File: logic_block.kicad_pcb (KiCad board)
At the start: 2 copper layers, 40 x 40 mm, 33 parts, among them J301 PogoPin, J302 PogoPin, J303 PogoPin, J304 PogoPin, J305 PogoPin, J306 PogoPin, J307 WritePad, Q301 NMOS, Q302 NMOS, Q303 NMOS, Q304 NMOS, U301 ATtiny404-SS

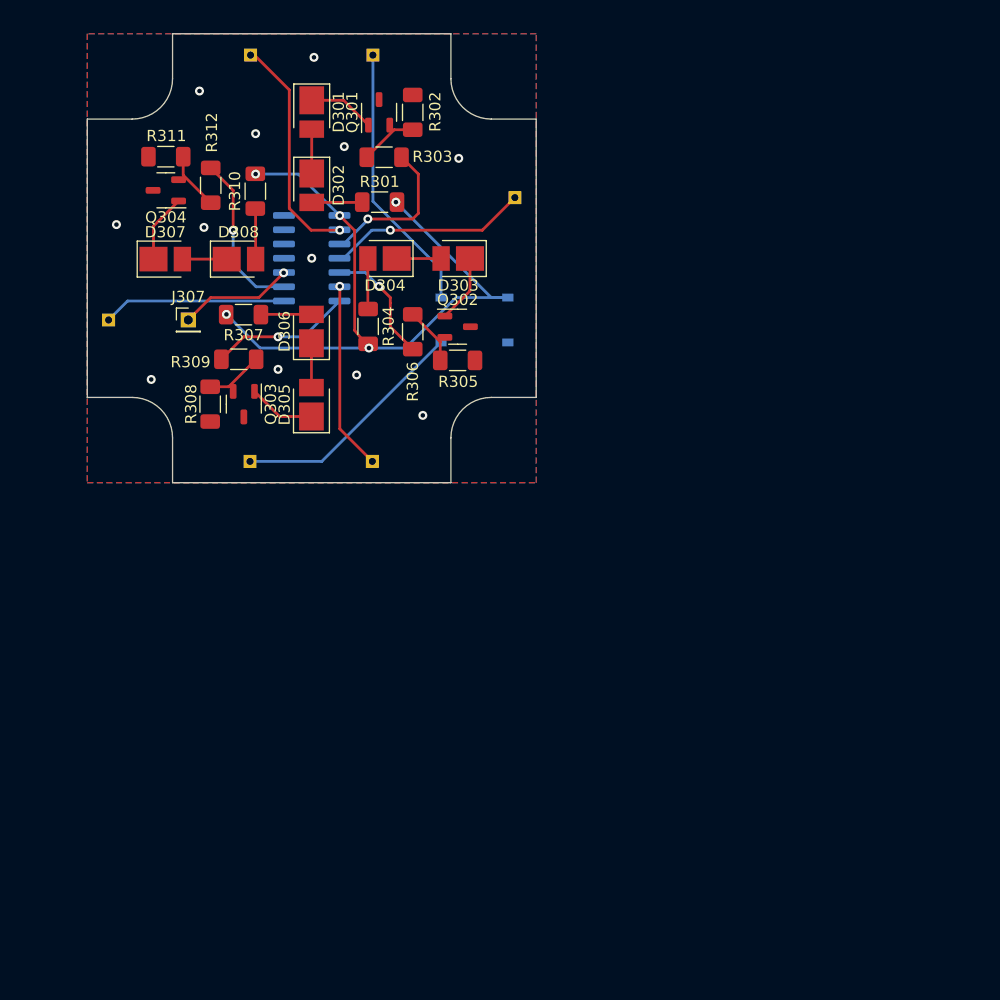
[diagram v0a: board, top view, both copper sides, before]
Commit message: gerber
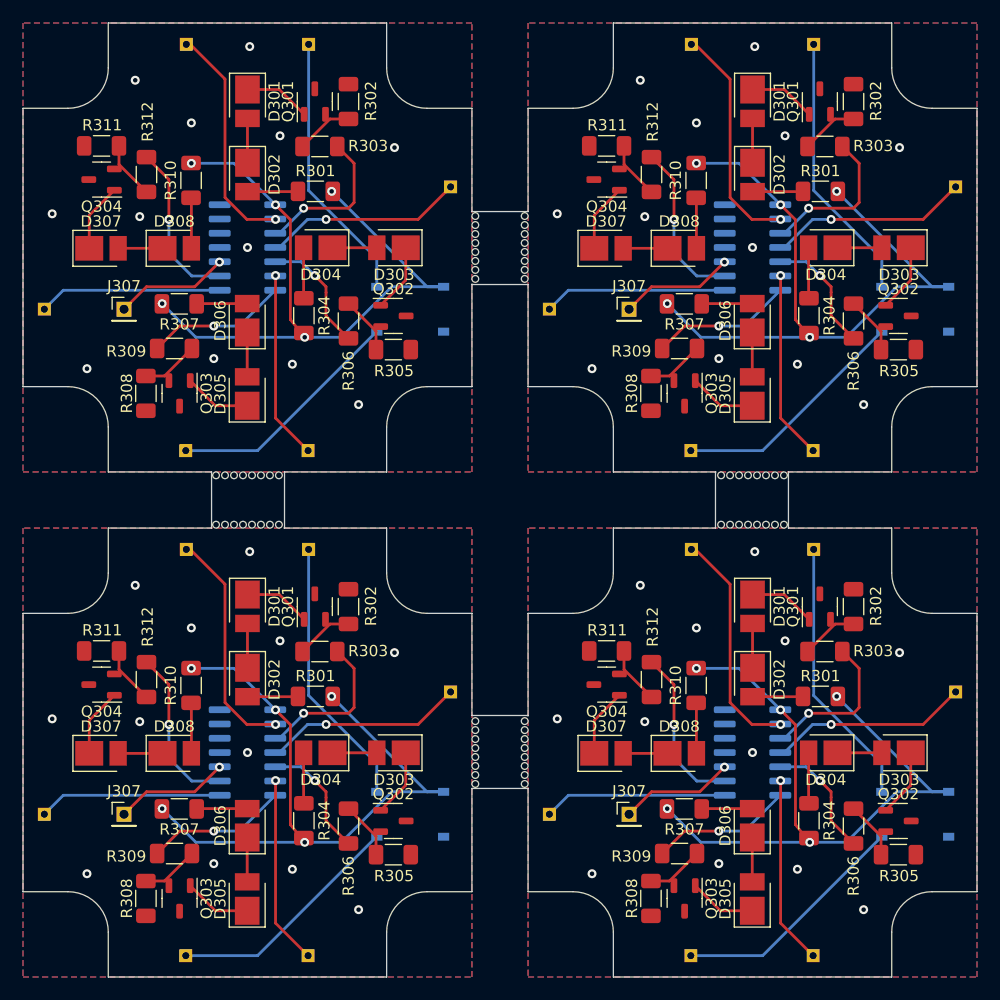
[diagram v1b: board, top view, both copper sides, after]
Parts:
- removed the D301 at (120.0, 57.0)
- removed the D302 at (120.0, 63.5)
- removed the D303 at (133.1, 70.0)
- removed the D304 at (126.5, 70.0)
- removed the D305 at (120.0, 83.0)
- removed the D306 at (120.0, 76.5)
- removed the D307 at (107.0, 70.1)
- removed the D308 at (113.5, 70.1)
- removed the D309 at (134.5, 75.5)
- removed the J301 at (114.5, 51.9)
- removed the J302 at (138.1, 64.6)
- removed the J303 at (125.4, 88.1)
- removed the J304 at (101.9, 75.5)
- removed the J305 at (125.5, 51.9)
- removed the J306 at (114.5, 88.1)
- removed the J307 at (109.0, 75.5)
- removed the Q301 at (126.0, 57.0)
- removed the Q302 at (133.0, 76.1)
- removed the Q303 at (114.0, 83.0)
- removed the Q304 at (107.0, 64.0)
- removed the R301 at (126.0, 65.0)
- removed the R302 at (129.0, 57.0)
- removed the R303 at (126.5, 61.0)
- removed the R304 at (125.0, 76.1)
- removed the R305 at (133.0, 79.1)
- removed the R306 at (129.0, 76.5)
- removed the R307 at (113.9, 75.0)
- removed the R308 at (111.0, 83.0)
- removed the R309 at (113.5, 79.0)
- removed the R310 at (115.0, 64.0)
- removed the R311 at (107.0, 61.0)
- removed the R312 at (111.0, 63.5)
- removed the U301 at (120.0, 70.0)
- added D301: LED, LED_SMD:LED_PLCC_2835_Handsoldering, F.Cu at (114.3, 56.0)
- added D301: LED, LED_SMD:LED_PLCC_2835_Handsoldering, F.Cu at (114.3, 101.0)
- added D301: LED, LED_SMD:LED_PLCC_2835_Handsoldering, F.Cu at (159.3, 56.0)
- added D301: LED, LED_SMD:LED_PLCC_2835_Handsoldering, F.Cu at (159.3, 101.0)
- added D302: LED, LED_SMD:LED_PLCC_2835_Handsoldering, F.Cu at (159.3, 62.5)
- added D302: LED, LED_SMD:LED_PLCC_2835_Handsoldering, F.Cu at (114.3, 107.5)
- added D302: LED, LED_SMD:LED_PLCC_2835_Handsoldering, F.Cu at (114.3, 62.5)
- added D302: LED, LED_SMD:LED_PLCC_2835_Handsoldering, F.Cu at (159.3, 107.5)
- added D303: LED, LED_SMD:LED_PLCC_2835_Handsoldering, F.Cu at (172.3, 69.1)
- added D303: LED, LED_SMD:LED_PLCC_2835_Handsoldering, F.Cu at (127.3, 69.1)
- added D303: LED, LED_SMD:LED_PLCC_2835_Handsoldering, F.Cu at (127.3, 114.1)
- added D303: LED, LED_SMD:LED_PLCC_2835_Handsoldering, F.Cu at (172.3, 114.1)
- added D304: LED, LED_SMD:LED_PLCC_2835_Handsoldering, F.Cu at (165.8, 114.1)
- added D304: LED, LED_SMD:LED_PLCC_2835_Handsoldering, F.Cu at (120.8, 114.1)
- added D304: LED, LED_SMD:LED_PLCC_2835_Handsoldering, F.Cu at (165.8, 69.1)
- added D304: LED, LED_SMD:LED_PLCC_2835_Handsoldering, F.Cu at (120.8, 69.1)
- added D305: LED, LED_SMD:LED_PLCC_2835_Handsoldering, F.Cu at (159.2, 82.1)
- added D305: LED, LED_SMD:LED_PLCC_2835_Handsoldering, F.Cu at (159.2, 127.1)
- added D305: LED, LED_SMD:LED_PLCC_2835_Handsoldering, F.Cu at (114.2, 82.1)
- added D305: LED, LED_SMD:LED_PLCC_2835_Handsoldering, F.Cu at (114.2, 127.1)
- added D306: LED, LED_SMD:LED_PLCC_2835_Handsoldering, F.Cu at (159.2, 120.6)
- added D306: LED, LED_SMD:LED_PLCC_2835_Handsoldering, F.Cu at (159.2, 75.6)
- added D306: LED, LED_SMD:LED_PLCC_2835_Handsoldering, F.Cu at (114.2, 75.6)
- added D306: LED, LED_SMD:LED_PLCC_2835_Handsoldering, F.Cu at (114.2, 120.6)
- added D307: LED, LED_SMD:LED_PLCC_2835_Handsoldering, F.Cu at (101.2, 69.1)
- added D307: LED, LED_SMD:LED_PLCC_2835_Handsoldering, F.Cu at (146.2, 69.1)
- added D307: LED, LED_SMD:LED_PLCC_2835_Handsoldering, F.Cu at (101.2, 114.1)
- added D307: LED, LED_SMD:LED_PLCC_2835_Handsoldering, F.Cu at (146.2, 114.1)
- added D308: LED, LED_SMD:LED_PLCC_2835_Handsoldering, F.Cu at (107.8, 114.1)
- added D308: LED, LED_SMD:LED_PLCC_2835_Handsoldering, F.Cu at (152.8, 114.1)
- added D308: LED, LED_SMD:LED_PLCC_2835_Handsoldering, F.Cu at (107.8, 69.1)
- added D308: LED, LED_SMD:LED_PLCC_2835_Handsoldering, F.Cu at (152.8, 69.1)
- added D309: ABS2, Diode_SMD:Diode_Bridge_Diotec_ABS, B.Cu at (173.8, 74.5)
- added D309: ABS2, Diode_SMD:Diode_Bridge_Diotec_ABS, B.Cu at (128.8, 74.5)
- added D309: ABS2, Diode_SMD:Diode_Bridge_Diotec_ABS, B.Cu at (173.8, 119.5)
- added D309: ABS2, Diode_SMD:Diode_Bridge_Diotec_ABS, B.Cu at (128.8, 119.5)
- added J301: PogoPin, LIB:0906015207614110, B.Cu at (108.8, 50.9)
- added J301: PogoPin, LIB:0906015207614110, B.Cu at (108.8, 95.9)
- added J301: PogoPin, LIB:0906015207614110, B.Cu at (153.8, 50.9)
- added J301: PogoPin, LIB:0906015207614110, B.Cu at (153.8, 95.9)
- added J302: PogoPin, LIB:0906015207614110, B.Cu at (177.4, 108.6)
- added J302: PogoPin, LIB:0906015207614110, B.Cu at (132.4, 63.6)
- added J302: PogoPin, LIB:0906015207614110, B.Cu at (177.4, 63.6)
- added J302: PogoPin, LIB:0906015207614110, B.Cu at (132.4, 108.6)
- added J303: PogoPin, LIB:0906015207614110, B.Cu at (119.7, 132.1)
- added J303: PogoPin, LIB:0906015207614110, B.Cu at (164.7, 132.1)
- added J303: PogoPin, LIB:0906015207614110, B.Cu at (164.7, 87.1)
- added J303: PogoPin, LIB:0906015207614110, B.Cu at (119.7, 87.1)
- added J304: PogoPin, LIB:0906015207614110, B.Cu at (96.2, 119.5)
- added J304: PogoPin, LIB:0906015207614110, B.Cu at (96.2, 74.5)
- added J304: PogoPin, LIB:0906015207614110, B.Cu at (141.2, 74.5)
- added J304: PogoPin, LIB:0906015207614110, B.Cu at (141.2, 119.5)
- added J305: PogoPin, LIB:0906015207614110, B.Cu at (164.7, 50.9)
- added J305: PogoPin, LIB:0906015207614110, B.Cu at (119.7, 50.9)
- added J305: PogoPin, LIB:0906015207614110, B.Cu at (164.7, 95.9)
- added J305: PogoPin, LIB:0906015207614110, B.Cu at (119.7, 95.9)
- added J306: PogoPin, LIB:0906015207614110, B.Cu at (153.8, 132.1)
- added J306: PogoPin, LIB:0906015207614110, B.Cu at (153.8, 87.1)
- added J306: PogoPin, LIB:0906015207614110, B.Cu at (108.8, 87.1)
- added J306: PogoPin, LIB:0906015207614110, B.Cu at (108.8, 132.1)
- added J307: WritePad, Connector_PinHeader_2.00mm:PinHeader_1x01_P2.00mm_Vertical, F.Cu at (103.3, 74.5)
- added J307: WritePad, Connector_PinHeader_2.00mm:PinHeader_1x01_P2.00mm_Vertical, F.Cu at (148.3, 119.5)
- added J307: WritePad, Connector_PinHeader_2.00mm:PinHeader_1x01_P2.00mm_Vertical, F.Cu at (148.3, 74.5)
- added J307: WritePad, Connector_PinHeader_2.00mm:PinHeader_1x01_P2.00mm_Vertical, F.Cu at (103.3, 119.5)
- added Q301: NMOS, Package_TO_SOT_SMD:SOT-23-3, F.Cu at (120.3, 101.0)
- added Q301: NMOS, Package_TO_SOT_SMD:SOT-23-3, F.Cu at (165.3, 56.0)
- added Q301: NMOS, Package_TO_SOT_SMD:SOT-23-3, F.Cu at (165.3, 101.0)
- added Q301: NMOS, Package_TO_SOT_SMD:SOT-23-3, F.Cu at (120.3, 56.0)
- added Q302: NMOS, Package_TO_SOT_SMD:SOT-23-3, F.Cu at (127.3, 120.1)
- added Q302: NMOS, Package_TO_SOT_SMD:SOT-23-3, F.Cu at (172.3, 75.1)
- added Q302: NMOS, Package_TO_SOT_SMD:SOT-23-3, F.Cu at (127.3, 75.1)
- added Q302: NMOS, Package_TO_SOT_SMD:SOT-23-3, F.Cu at (172.3, 120.1)
- added Q303: NMOS, Package_TO_SOT_SMD:SOT-23-3, F.Cu at (108.2, 82.0)
- added Q303: NMOS, Package_TO_SOT_SMD:SOT-23-3, F.Cu at (153.2, 82.0)
- added Q303: NMOS, Package_TO_SOT_SMD:SOT-23-3, F.Cu at (153.2, 127.0)
- added Q303: NMOS, Package_TO_SOT_SMD:SOT-23-3, F.Cu at (108.2, 127.0)
- added Q304: NMOS, Package_TO_SOT_SMD:SOT-23-3, F.Cu at (101.3, 108.0)
- added Q304: NMOS, Package_TO_SOT_SMD:SOT-23-3, F.Cu at (101.3, 63.0)
- added Q304: NMOS, Package_TO_SOT_SMD:SOT-23-3, F.Cu at (146.3, 63.0)
- added Q304: NMOS, Package_TO_SOT_SMD:SOT-23-3, F.Cu at (146.3, 108.0)
- added R301: 47Ω, Resistor_SMD:R_1206_3216Metric_Pad1.30x1.75mm_HandSolder, F.Cu at (165.3, 64.0)
- added R301: 47Ω, Resistor_SMD:R_1206_3216Metric_Pad1.30x1.75mm_HandSolder, F.Cu at (165.3, 109.0)
- added R301: 47Ω, Resistor_SMD:R_1206_3216Metric_Pad1.30x1.75mm_HandSolder, F.Cu at (120.3, 64.0)
- added R301: 47Ω, Resistor_SMD:R_1206_3216Metric_Pad1.30x1.75mm_HandSolder, F.Cu at (120.3, 109.0)
- added R302: 10kΩ, Resistor_SMD:R_1206_3216Metric_Pad1.30x1.75mm_HandSolder, F.Cu at (168.3, 101.0)
- added R302: 10kΩ, Resistor_SMD:R_1206_3216Metric_Pad1.30x1.75mm_HandSolder, F.Cu at (123.3, 56.0)
- added R302: 10kΩ, Resistor_SMD:R_1206_3216Metric_Pad1.30x1.75mm_HandSolder, F.Cu at (123.3, 101.0)
- added R302: 10kΩ, Resistor_SMD:R_1206_3216Metric_Pad1.30x1.75mm_HandSolder, F.Cu at (168.3, 56.0)
- added R303: 100Ω, Resistor_SMD:R_1206_3216Metric_Pad1.30x1.75mm_HandSolder, F.Cu at (165.7, 105.0)
- added R303: 100Ω, Resistor_SMD:R_1206_3216Metric_Pad1.30x1.75mm_HandSolder, F.Cu at (120.7, 105.0)
- added R303: 100Ω, Resistor_SMD:R_1206_3216Metric_Pad1.30x1.75mm_HandSolder, F.Cu at (120.7, 60.0)
- added R303: 100Ω, Resistor_SMD:R_1206_3216Metric_Pad1.30x1.75mm_HandSolder, F.Cu at (165.7, 60.0)
- added R304: 47Ω, Resistor_SMD:R_1206_3216Metric_Pad1.30x1.75mm_HandSolder, F.Cu at (119.3, 75.1)
- added R304: 47Ω, Resistor_SMD:R_1206_3216Metric_Pad1.30x1.75mm_HandSolder, F.Cu at (164.3, 75.1)
- added R304: 47Ω, Resistor_SMD:R_1206_3216Metric_Pad1.30x1.75mm_HandSolder, F.Cu at (164.3, 120.1)
- added R304: 47Ω, Resistor_SMD:R_1206_3216Metric_Pad1.30x1.75mm_HandSolder, F.Cu at (119.3, 120.1)
- added R305: 10kΩ, Resistor_SMD:R_1206_3216Metric_Pad1.30x1.75mm_HandSolder, F.Cu at (127.3, 78.1)
- added R305: 10kΩ, Resistor_SMD:R_1206_3216Metric_Pad1.30x1.75mm_HandSolder, F.Cu at (172.3, 78.1)
- added R305: 10kΩ, Resistor_SMD:R_1206_3216Metric_Pad1.30x1.75mm_HandSolder, F.Cu at (172.3, 123.1)
- added R305: 10kΩ, Resistor_SMD:R_1206_3216Metric_Pad1.30x1.75mm_HandSolder, F.Cu at (127.3, 123.1)
- added R306: 100Ω, Resistor_SMD:R_1206_3216Metric_Pad1.30x1.75mm_HandSolder, F.Cu at (123.3, 75.6)
- added R306: 100Ω, Resistor_SMD:R_1206_3216Metric_Pad1.30x1.75mm_HandSolder, F.Cu at (168.3, 75.6)
- added R306: 100Ω, Resistor_SMD:R_1206_3216Metric_Pad1.30x1.75mm_HandSolder, F.Cu at (168.3, 120.6)
- added R306: 100Ω, Resistor_SMD:R_1206_3216Metric_Pad1.30x1.75mm_HandSolder, F.Cu at (123.3, 120.6)
- added R307: 47Ω, Resistor_SMD:R_1206_3216Metric_Pad1.30x1.75mm_HandSolder, F.Cu at (153.2, 74.1)
- added R307: 47Ω, Resistor_SMD:R_1206_3216Metric_Pad1.30x1.75mm_HandSolder, F.Cu at (153.2, 119.1)
- added R307: 47Ω, Resistor_SMD:R_1206_3216Metric_Pad1.30x1.75mm_HandSolder, F.Cu at (108.2, 74.1)
- added R307: 47Ω, Resistor_SMD:R_1206_3216Metric_Pad1.30x1.75mm_HandSolder, F.Cu at (108.2, 119.1)
- added R308: 10kΩ, Resistor_SMD:R_1206_3216Metric_Pad1.30x1.75mm_HandSolder, F.Cu at (105.2, 127.0)
- added R308: 10kΩ, Resistor_SMD:R_1206_3216Metric_Pad1.30x1.75mm_HandSolder, F.Cu at (150.2, 82.0)
- added R308: 10kΩ, Resistor_SMD:R_1206_3216Metric_Pad1.30x1.75mm_HandSolder, F.Cu at (150.2, 127.0)
- added R308: 10kΩ, Resistor_SMD:R_1206_3216Metric_Pad1.30x1.75mm_HandSolder, F.Cu at (105.2, 82.0)
- added R309: 100Ω, Resistor_SMD:R_1206_3216Metric_Pad1.30x1.75mm_HandSolder, F.Cu at (107.8, 123.0)
- added R309: 100Ω, Resistor_SMD:R_1206_3216Metric_Pad1.30x1.75mm_HandSolder, F.Cu at (152.8, 78.0)
- added R309: 100Ω, Resistor_SMD:R_1206_3216Metric_Pad1.30x1.75mm_HandSolder, F.Cu at (152.8, 123.0)
- added R309: 100Ω, Resistor_SMD:R_1206_3216Metric_Pad1.30x1.75mm_HandSolder, F.Cu at (107.8, 78.0)
- added R310: 47Ω, Resistor_SMD:R_1206_3216Metric_Pad1.30x1.75mm_HandSolder, F.Cu at (109.2, 63.1)
- added R310: 47Ω, Resistor_SMD:R_1206_3216Metric_Pad1.30x1.75mm_HandSolder, F.Cu at (109.2, 108.1)
- added R310: 47Ω, Resistor_SMD:R_1206_3216Metric_Pad1.30x1.75mm_HandSolder, F.Cu at (154.2, 108.1)
- added R310: 47Ω, Resistor_SMD:R_1206_3216Metric_Pad1.30x1.75mm_HandSolder, F.Cu at (154.2, 63.1)
- added R311: 10kΩ, Resistor_SMD:R_1206_3216Metric_Pad1.30x1.75mm_HandSolder, F.Cu at (101.3, 105.0)
- added R311: 10kΩ, Resistor_SMD:R_1206_3216Metric_Pad1.30x1.75mm_HandSolder, F.Cu at (146.3, 60.0)
- added R311: 10kΩ, Resistor_SMD:R_1206_3216Metric_Pad1.30x1.75mm_HandSolder, F.Cu at (146.3, 105.0)
- added R311: 10kΩ, Resistor_SMD:R_1206_3216Metric_Pad1.30x1.75mm_HandSolder, F.Cu at (101.3, 60.0)
- added R312: 100Ω, Resistor_SMD:R_1206_3216Metric_Pad1.30x1.75mm_HandSolder, F.Cu at (105.3, 62.5)
- added R312: 100Ω, Resistor_SMD:R_1206_3216Metric_Pad1.30x1.75mm_HandSolder, F.Cu at (150.3, 107.5)
- added R312: 100Ω, Resistor_SMD:R_1206_3216Metric_Pad1.30x1.75mm_HandSolder, F.Cu at (105.3, 107.5)
- added R312: 100Ω, Resistor_SMD:R_1206_3216Metric_Pad1.30x1.75mm_HandSolder, F.Cu at (150.3, 62.5)
- added REF**: bridge, LIB:bridge, F.Cu at (162.5, 94.0)
- added REF**: bridge, LIB:bridge, F.Cu at (134.3, 117.2)
- added REF**: bridge, LIB:bridge, F.Cu at (111.1, 89.0)
- added REF**: bridge, LIB:bridge, F.Cu at (139.3, 65.8)
- added U301: ATtiny404-SS, Package_SO:SOIC-14_3.9x8.7mm_P1.27mm, B.Cu at (159.3, 69.0)
- added U301: ATtiny404-SS, Package_SO:SOIC-14_3.9x8.7mm_P1.27mm, B.Cu at (159.3, 114.0)
- added U301: ATtiny404-SS, Package_SO:SOIC-14_3.9x8.7mm_P1.27mm, B.Cu at (114.3, 69.0)
- added U301: ATtiny404-SS, Package_SO:SOIC-14_3.9x8.7mm_P1.27mm, B.Cu at (114.3, 114.0)
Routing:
- net +5V: track 63.9 -> 255.6 mm, vias 5 -> 20
- net Net-(J305-Pin_1): track 24.1 -> 96.5 mm
- net Net-(J306-Pin_1): track 21.4 -> 85.7 mm
- net N_S: track 20.6 -> 82.4 mm, vias 1 -> 4
- net E_S: track 17.9 -> 71.4 mm, vias 1 -> 4
- net S_S: track 16.8 -> 67.2 mm, vias 1 -> 4
- net W_S: track 16.3 -> 65.3 mm
- net W_LED: track 14.7 -> 59.0 mm, vias 1 -> 4
- net N_LED: track 13.8 -> 55.3 mm, vias 1 -> 4
- net S_LED: track 12.7 -> 50.7 mm, vias 1 -> 4
- net E_LED: track 10.9 -> 43.5 mm, vias 1 -> 4
- net UPDI: track 10.2 -> 41.0 mm, vias 1 -> 4
- net Net-(D307-K): track 6.10 -> 24.4 mm
- net Net-(D303-K): track 6.05 -> 24.2 mm
- net Net-(D305-K): track 6.00 -> 24.0 mm
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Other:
- board size 40 x 40 mm -> 85 x 85 mm
